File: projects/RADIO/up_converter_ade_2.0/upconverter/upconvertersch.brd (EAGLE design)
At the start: 75 x 110 mm, 33 parts, among them IC1 ADE-1+, IC2 LD1117STR, J1 USB-A-S-S-B-TH

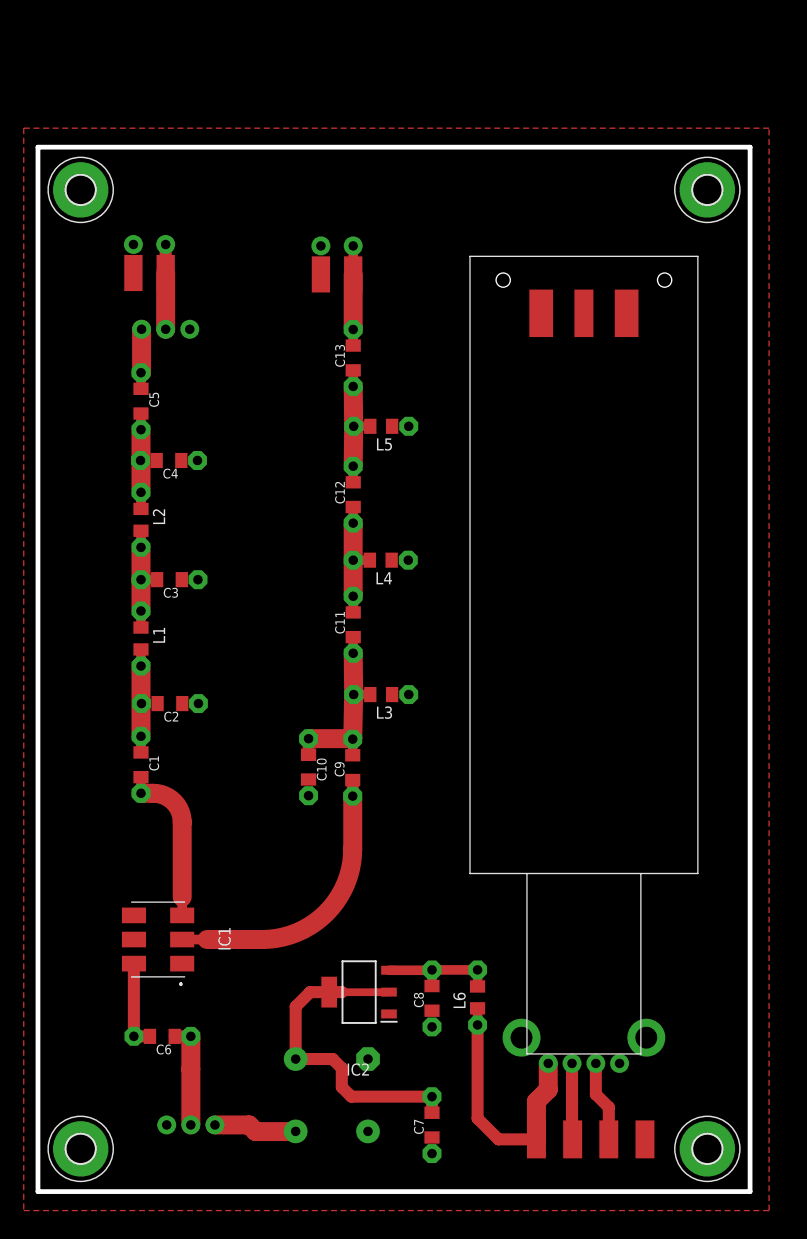
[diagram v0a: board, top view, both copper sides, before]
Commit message: update
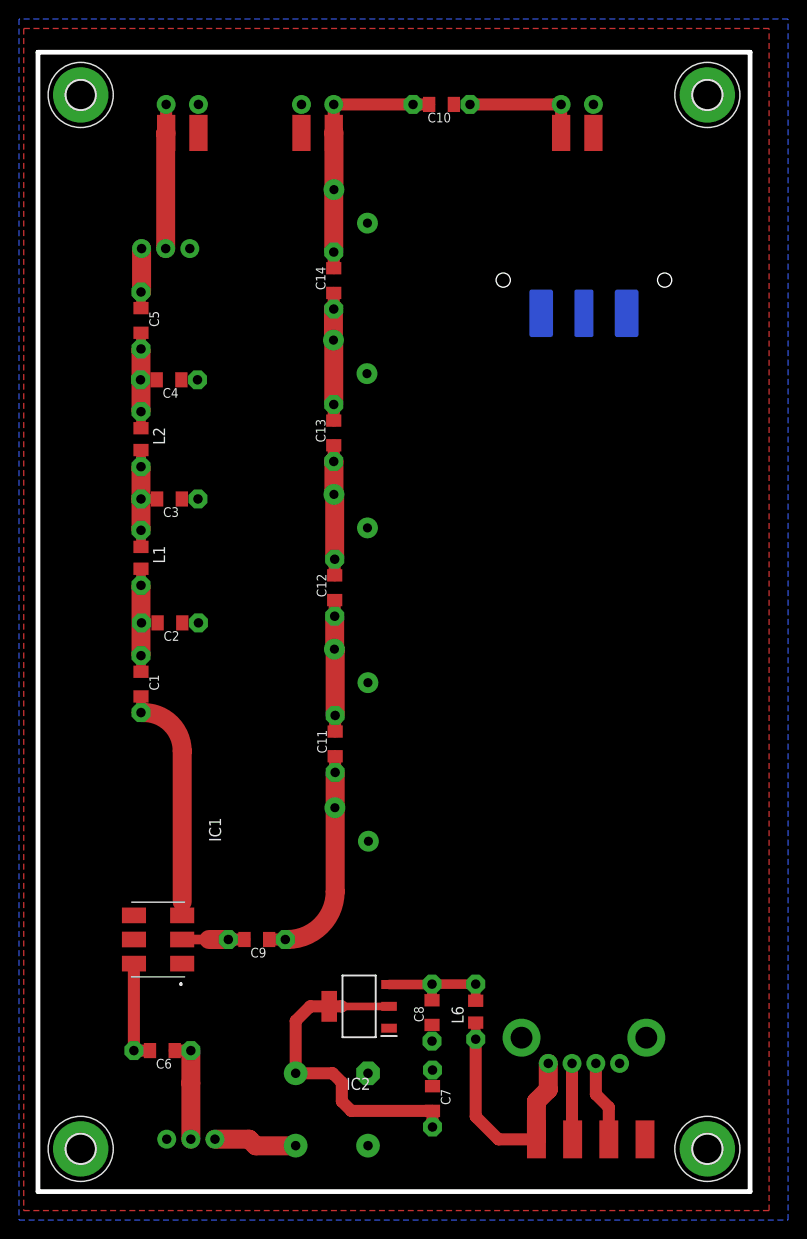
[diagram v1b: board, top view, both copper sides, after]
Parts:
- added C14: 56pF, mylib:C0805K
- added L7: 56nH, 164-11A06L:16411A06L
- added L8: 82nH, 164-11A06L:16411A06L
- added RF_OUT_VHF: 2X_SMD_PTH_PIN, mylib:2X_SMD_PTH
- C10: value 12pF -> 100pF
- C11: value 15pF -> 56pF
- C12: value 15pF -> 47pF
- C13: value 33pF -> 47pF
- C9: value 100pF -> 10nF
- L3: value 39nH -> 82nH; device mylib:M0805 -> 164-11A06L:16411A06L
- L4, L5: value 39nH -> 56nH; device mylib:M0805 -> 164-11A06L:16411A06L
- moved C10 71.2 mm to (42.5, 114.5), turned to 180 degrees
- moved C9 20.7 mm to (23.1, 26.6), turned to 180 degrees
- moved L3 15.5 mm to (34.8, 36.9), flipped to the bottom, turned to 0 degrees
- moved RF_IN 15.1 mm to (15.2, 111.5)
- moved RF_OUT 15.0 mm to (29.4, 111.5)
- moved L4 13.0 mm to (34.8, 53.6), flipped to the bottom, turned to 0 degrees
- moved C11 12.7 mm to (31.3, 47.1)
- moved L5 10.8 mm to (34.7, 69.9), flipped to the bottom, turned to 0 degrees
- moved H3 10.0 mm to (4.50, 115.5)
- moved H4 10.0 mm to (70.5, 115.5)
- moved C12 9.99 mm to (31.2, 63.6)
- moved C1 8.50 mm to (10.8, 53.5)
- moved C2 8.50 mm to (13.9, 59.9)
- moved C3 8.50 mm to (13.8, 73.0)
- moved C4 8.50 mm to (13.8, 85.5)
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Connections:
- new net N$14: C10.1, C10.P$1, RF_OUT_VHF.P$1, RF_OUT_VHF.T$1
- new net N$19: C13.2, C13.P$2, C14.1, C14.P$1, L7.2
- net GND: now also L7.1, L8.1, RF_IN.P$2, RF_IN.T$2, RF_OUT_VHF.P$2, RF_OUT_VHF.T$2; no longer C10.2, C10.P$2, L3.P$1, L4.P$1, L5.P$1, RF_IN.P$1, RF_IN.T$1
- net N$10: now also RF_IN.P$1, RF_IN.T$1; no longer RF_IN.P$2, RF_IN.T$2
- net N$15: now also C9.1, C9.P$1; no longer C10.1, C10.P$1, C9.2, C9.P$2, L3.P$2
- net N$16: no longer L4.P$2
- net N$17: no longer L5.P$2
- net N$18: now also C10.2, C10.P$2, C14.2, C14.P$2, L8.2; no longer C13.2, C13.P$2
- net N$2: now also C9.2, C9.P$2; no longer C9.1, C9.P$1
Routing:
- net N$2: track 29.2 -> 6.56 mm
- net N$18: track 10.5 -> 27.5 mm
- net N$19: track 0.00 -> 13.5 mm
- net N$14: track 0.00 -> 12.6 mm
- net N$1: track 17.1 -> 25.0 mm
- net N$10: track 8.93 -> 15.2 mm
- net N$15: track 20.6 -> 23.3 mm
- net N$3: track 9.37 -> 10.9 mm
- net N$12: track 27.2 -> 25.8 mm
- net N$16: track 12.8 -> 13.9 mm
- added copper zone on layer 16, net GND
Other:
- board size 75 x 110 mm -> 75 x 120 mm

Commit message: update
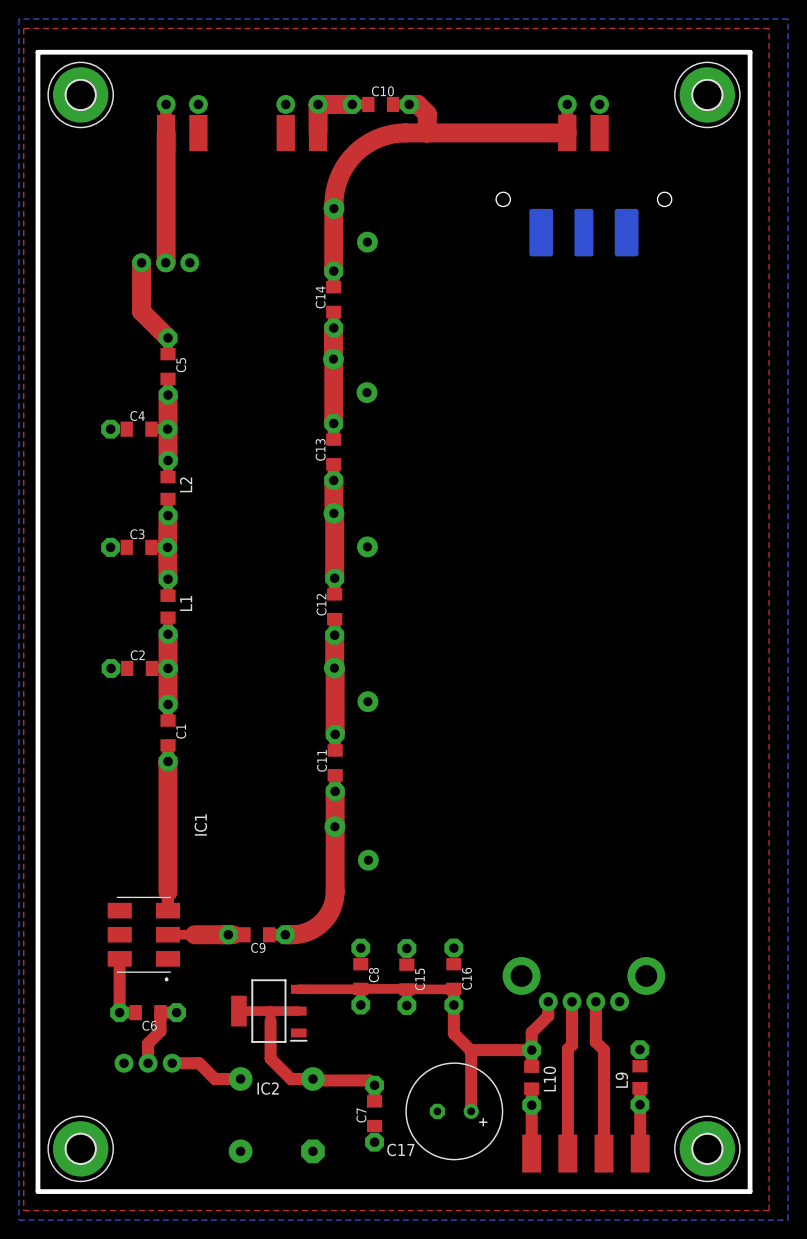
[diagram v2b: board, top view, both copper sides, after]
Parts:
- removed L6: 220uH, mylib:M0805
- removed RF_OUT_VHF: 2X_SMD_PTH_PIN, mylib:2X_SMD_PTH
- added C15, C16: 100nF, mylib:C0805K
- added C17: (no value), rcl:E3,5-10
- added L10, L9: 220uH, mylib:M0805
- added RF_IN_VHF: 2X_SMD_PTH_PIN, mylib:2X_SMD_PTH
- moved RF_OUT 28.0 mm to (57.5, 111.5)
- moved IC2 9.51 mm to (24.3, 19.0)
- moved R2 9.18 mm to (11.6, 12.2)
- moved U$1 8.50 mm to (45.5, 107.0)
- moved C8 8.41 mm to (34.0, 22.6), turned to 270 degrees
- moved J1 6.50 mm to (54.0, 20.0)
- moved C10 6.40 mm to (36.1, 114.5), turned to 0 degrees
- moved C7 6.31 mm to (35.5, 8.20), turned to 90 degrees
- moved C4 6.08 mm to (10.7, 80.3), turned to 0 degrees
- moved C3 6.02 mm to (10.7, 67.8), turned to 0 degrees
- moved C1 5.89 mm to (13.7, 48.3)
- moved L2 5.89 mm to (13.7, 74.1)
- moved L1 5.89 mm to (13.7, 61.6)
- moved QG1 5.83 mm to (25.1, 8.05), turned to 0 degrees
- moved C2 5.77 mm to (10.7, 55.1), turned to 0 degrees
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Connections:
- removed net N$14: C10.1, C10.P$1, RF_OUT_VHF.P$1, RF_OUT_VHF.T$1
- new net N$20: JH1.P$4, L9.1, L9.P$1
- new net N$21: JH1.P$1, L10.2, L10.P$2
- net GND: now also C15.1, C15.P$1, C16.1, C16.P$1, C17.-, L9.2, L9.P$2, RF_IN_VHF.P$1, RF_IN_VHF.T$1, RF_OUT.P$2, RF_OUT.T$2; no longer JH1.P$4, RF_OUT.P$1, RF_OUT.T$1, RF_OUT_VHF.P$2, RF_OUT_VHF.T$2
- net N$12: now also C10.1, C10.P$1, RF_IN_VHF.P$2, RF_IN_VHF.T$2; no longer J1.1, JH1.P$1, L6.1, L6.P$1
- net N$18: now also RF_OUT.P$1, RF_OUT.T$1; no longer RF_OUT.P$2, RF_OUT.T$2
- net VCC: now also C15.2, C15.P$2, C16.2, C16.P$2, C17.+, J1.1, L10.1, L10.P$1; no longer L6.2, L6.P$2
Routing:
- net VCC: track 12.6 -> 47.5 mm
- net N$18: track 27.5 -> 45.5 mm
- net N$12: track 25.8 -> 8.30 mm
- net N$14: track 12.6 -> 0.00 mm
- net 3.3V: track 34.9 -> 25.4 mm
- net N$4: track 8.03 -> 16.2 mm
- net N$5: track 8.57 -> 16.4 mm
- net N$1: track 25.0 -> 17.4 mm
- net N$20: track 0.00 -> 6.91 mm
- net N$21: track 0.00 -> 6.85 mm
- net N$6: track 10.8 -> 16.4 mm
- net N$9: track 6.29 -> 10.8 mm
- net N$8: track 10.0 -> 13.8 mm
- net N$3: track 10.9 -> 7.37 mm
- net N$13: track 11.0 -> 7.57 mm
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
